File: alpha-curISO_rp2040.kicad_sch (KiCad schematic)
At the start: 31 parts, among them U1 RP2040

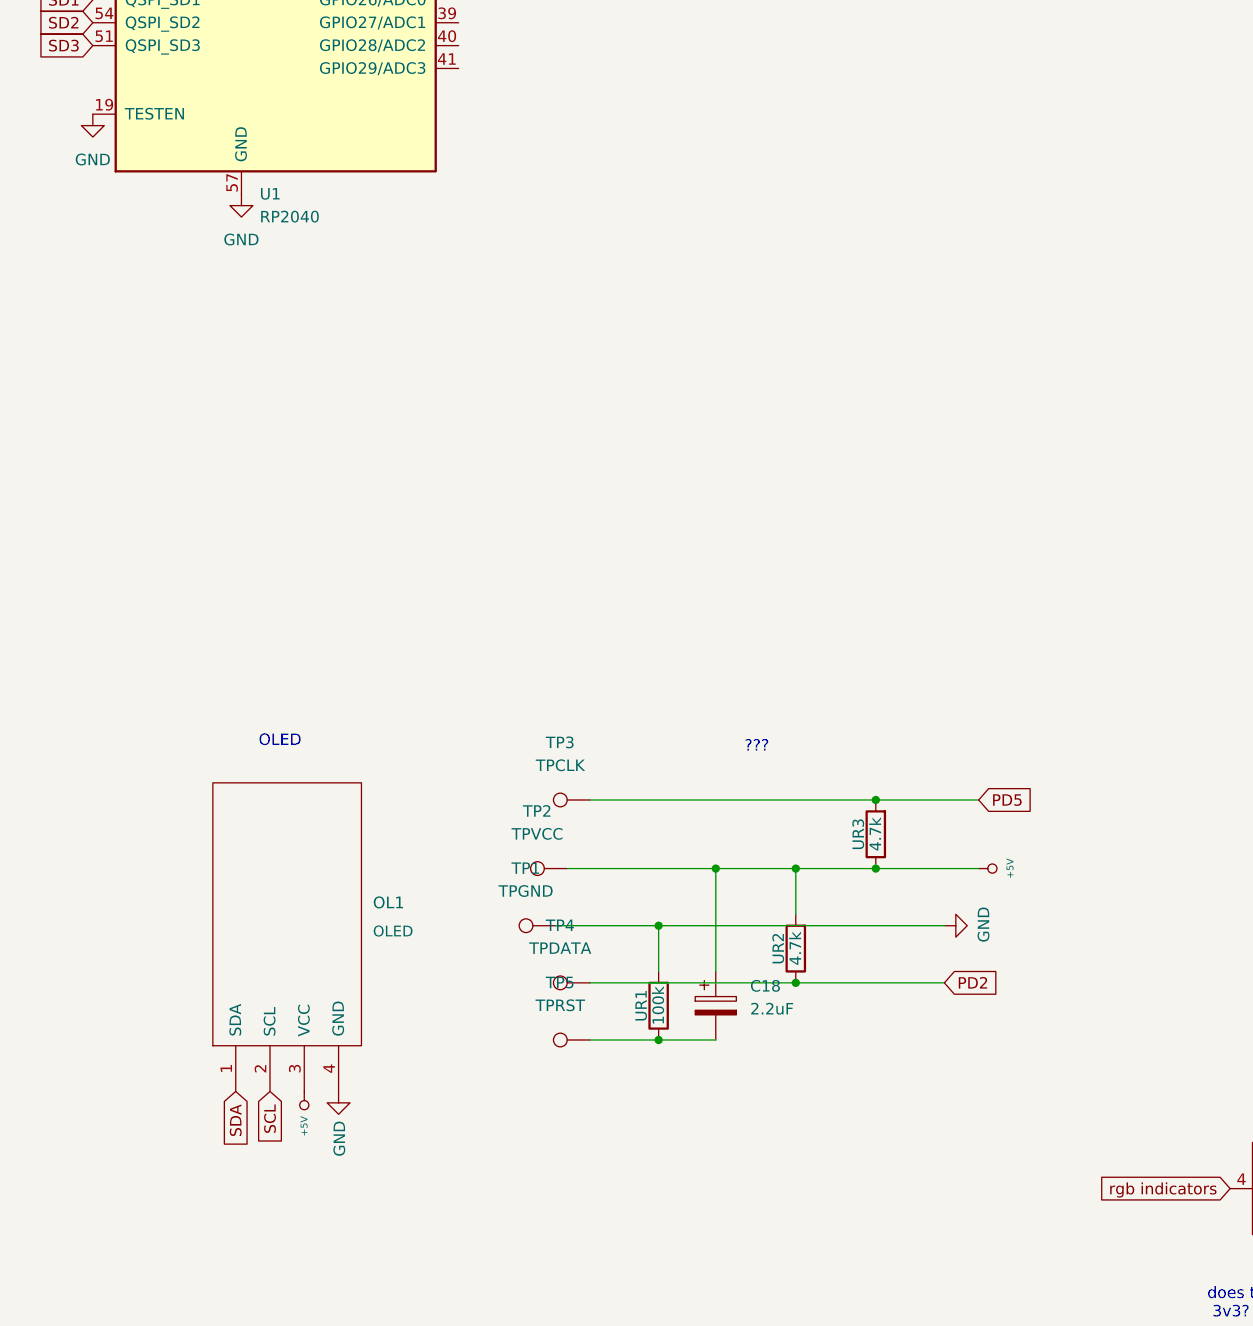
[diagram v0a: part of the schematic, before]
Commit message: galvy edits - start routing testing
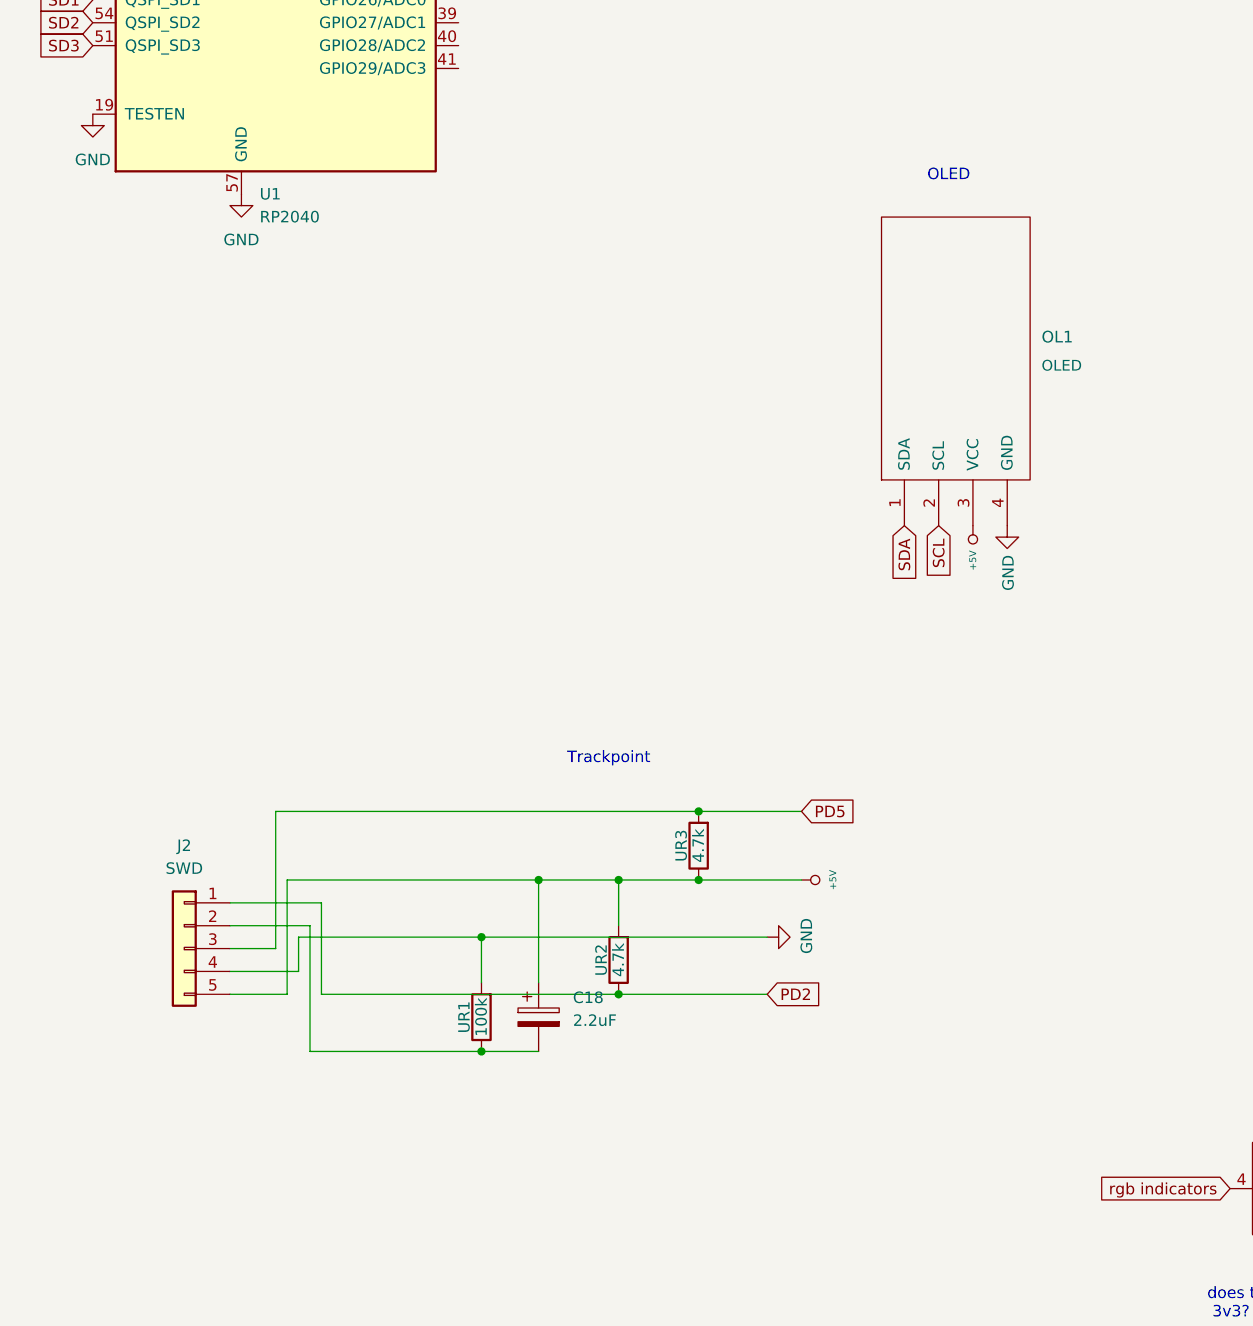
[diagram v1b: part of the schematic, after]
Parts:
- removed TP1: TPGND, TestPoint:TestPoint_THTPad_1.0x1.0mm_Drill0.5mm, symbol Connector:TestPoint
- removed TP2: TPVCC, TestPoint:TestPoint_THTPad_1.0x1.0mm_Drill0.5mm, symbol Connector:TestPoint
- removed TP3: TPCLK, TestPoint:TestPoint_THTPad_1.0x1.0mm_Drill0.5mm, symbol Connector:TestPoint
- removed TP4: TPDATA, TestPoint:TestPoint_THTPad_1.0x1.0mm_Drill0.5mm, symbol Connector:TestPoint
- removed TP5: TPRST, TestPoint:TestPoint_THTPad_1.0x1.0mm_Drill0.5mm, symbol Connector:TestPoint
- added J2: SWD, Connector_PinSocket_2.54mm:PinSocket_1x05_P2.54mm_Vertical, symbol Connector_Generic:Conn_01x05
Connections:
- net +5V: now also J2.5 (Pin_5)
- net GND: now also J2.4 (Pin_4)
- net PD2: now also J2.1 (Pin_1)
- net PD5: now also J2.3 (Pin_3)
- net at C18.2, UR1.1: now also J2.2 (Pin_2)
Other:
- note added: "Trackpoint"
- note removed: "???"
- moved on the sheet: C18, OL1, UR1, UR2, UR3
